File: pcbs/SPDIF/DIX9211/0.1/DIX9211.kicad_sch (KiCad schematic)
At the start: 67 parts, among them J1 Conn_01x02_Pin, J10 Conn_01x05_Pin, J11 Conn_01x04_Pin, J12 Conn_01x03_Pin, J13 Conn_01x02_Pin, J2 Conn_01x02_Pin, J3 Conn_01x02_Pin, J4 Conn_01x02_Pin, J5 Conn_01x02_Pin, J6 Conn_01x04_Pin, J7 Conn_01x04_Pin, J8 Conn_01x04_Pin, J9 Conn_01x02_Pin, U1 DA101C_C6931652, U2 DA101C_C6931652, U3 DA101C_C6931652, U4 DA101C_C6931652, U5 74HC7014, U6 DIX9211, U7 AMS1117-3.3, Y1 24.576MHz

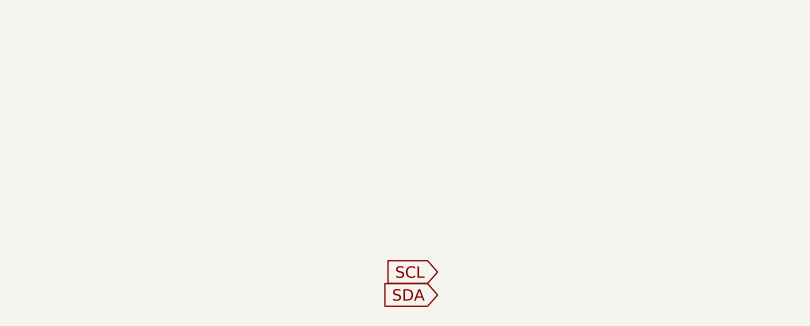
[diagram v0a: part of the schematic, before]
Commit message: Updates
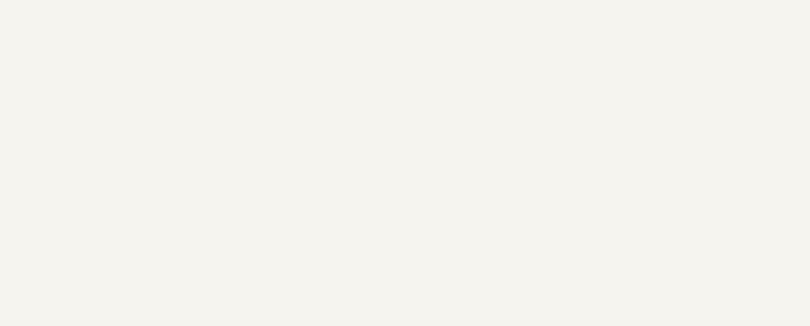
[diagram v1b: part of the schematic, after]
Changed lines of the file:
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@@
-		)
-	)
-	(global_label "SCL"
-		(shape input)
-		(at 274.32 293.37 180)
-		(fields_autoplaced yes)
-		(effects
-			(font
-				(size 1.27 1.27)
-			)
-			(justify right)
-		)
-		(property "Intersheetrefs" "${INTERSHEET_REFS}"
-			(at 267.8272 293.37 0)
-			(effects
-				(font
-					(size 1.27 1.27)
-				)
-				(justify right)
-				(hide yes)
-			)
 		)
 	)
@@
 				(hide yes)
 			)
-		)
-	)
-	(global_label "SDA"
-		(shape input)
-		(at 274.32 295.91 180)
-		(fields_autoplaced yes)
-		(effects
-			(font
-				(size 1.27 1.27)
-			)
-			(justify right)
-		)
-		(property "Intersheetrefs" "${INTERSHEET_REFS}"
-			(at 267.7667 295.91 0)
-			(effects
-				(font
-					(size 1.27 1.27)
-				)
-				(justify right)
-				(hide yes)
-			)
